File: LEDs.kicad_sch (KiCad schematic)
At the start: 62 parts, among them J5 Case Lighting

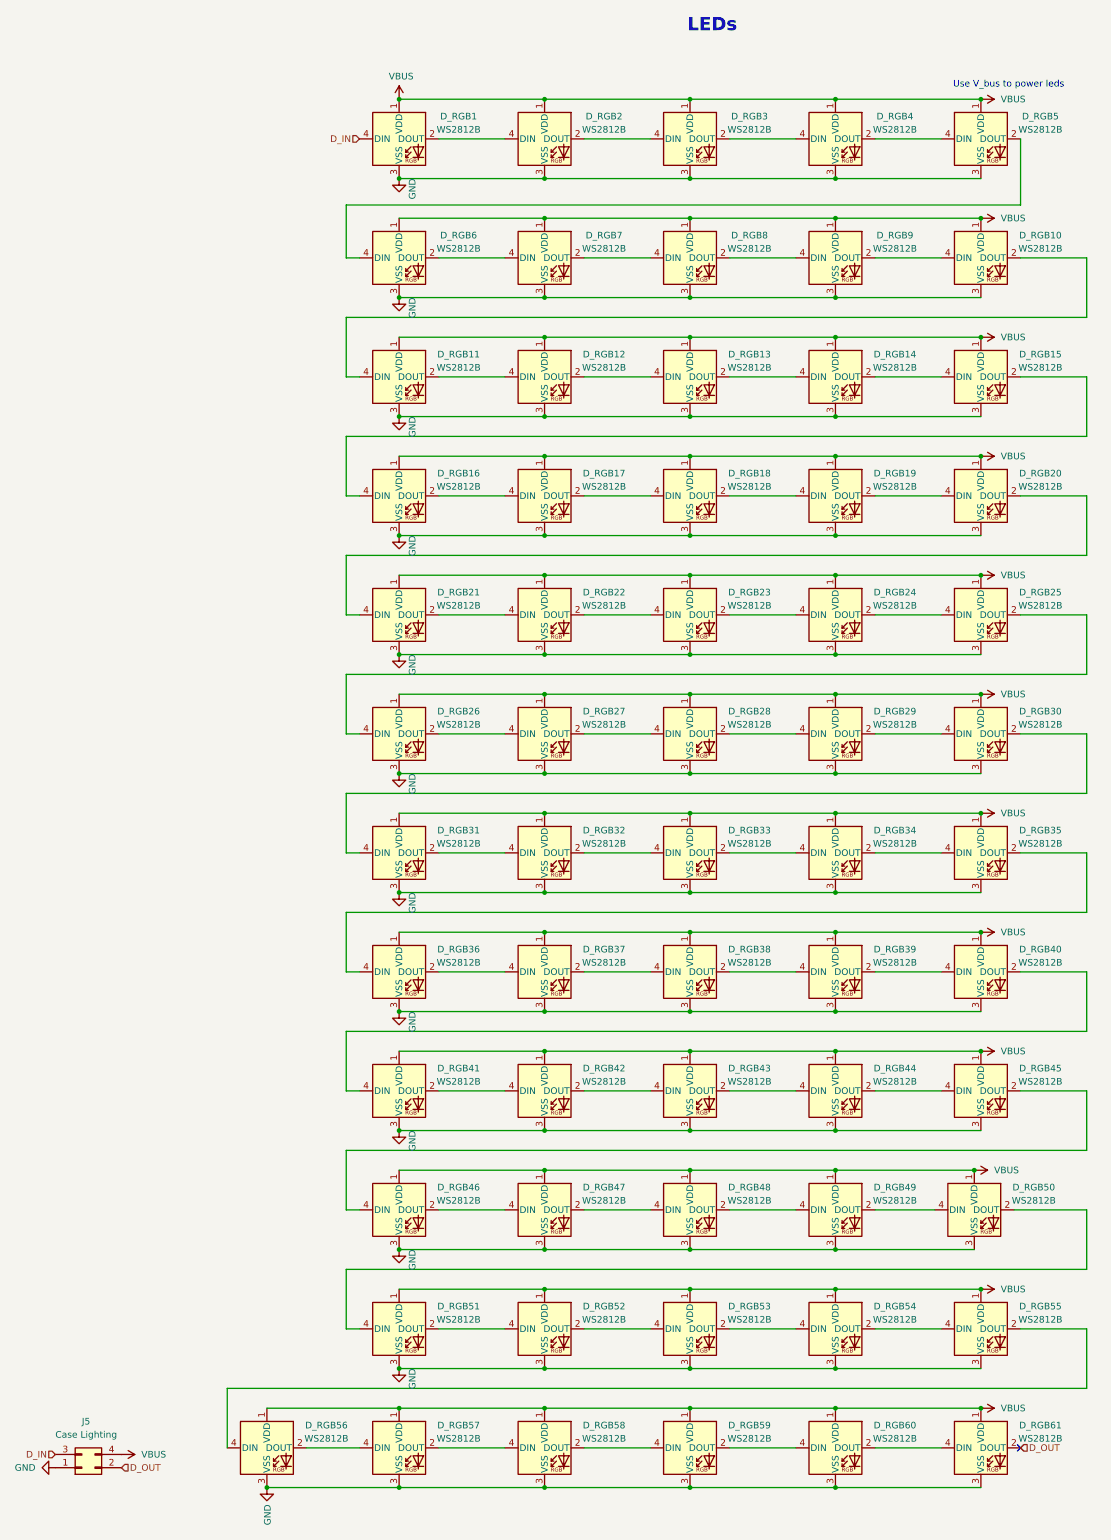
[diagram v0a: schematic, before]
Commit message: pretty much done
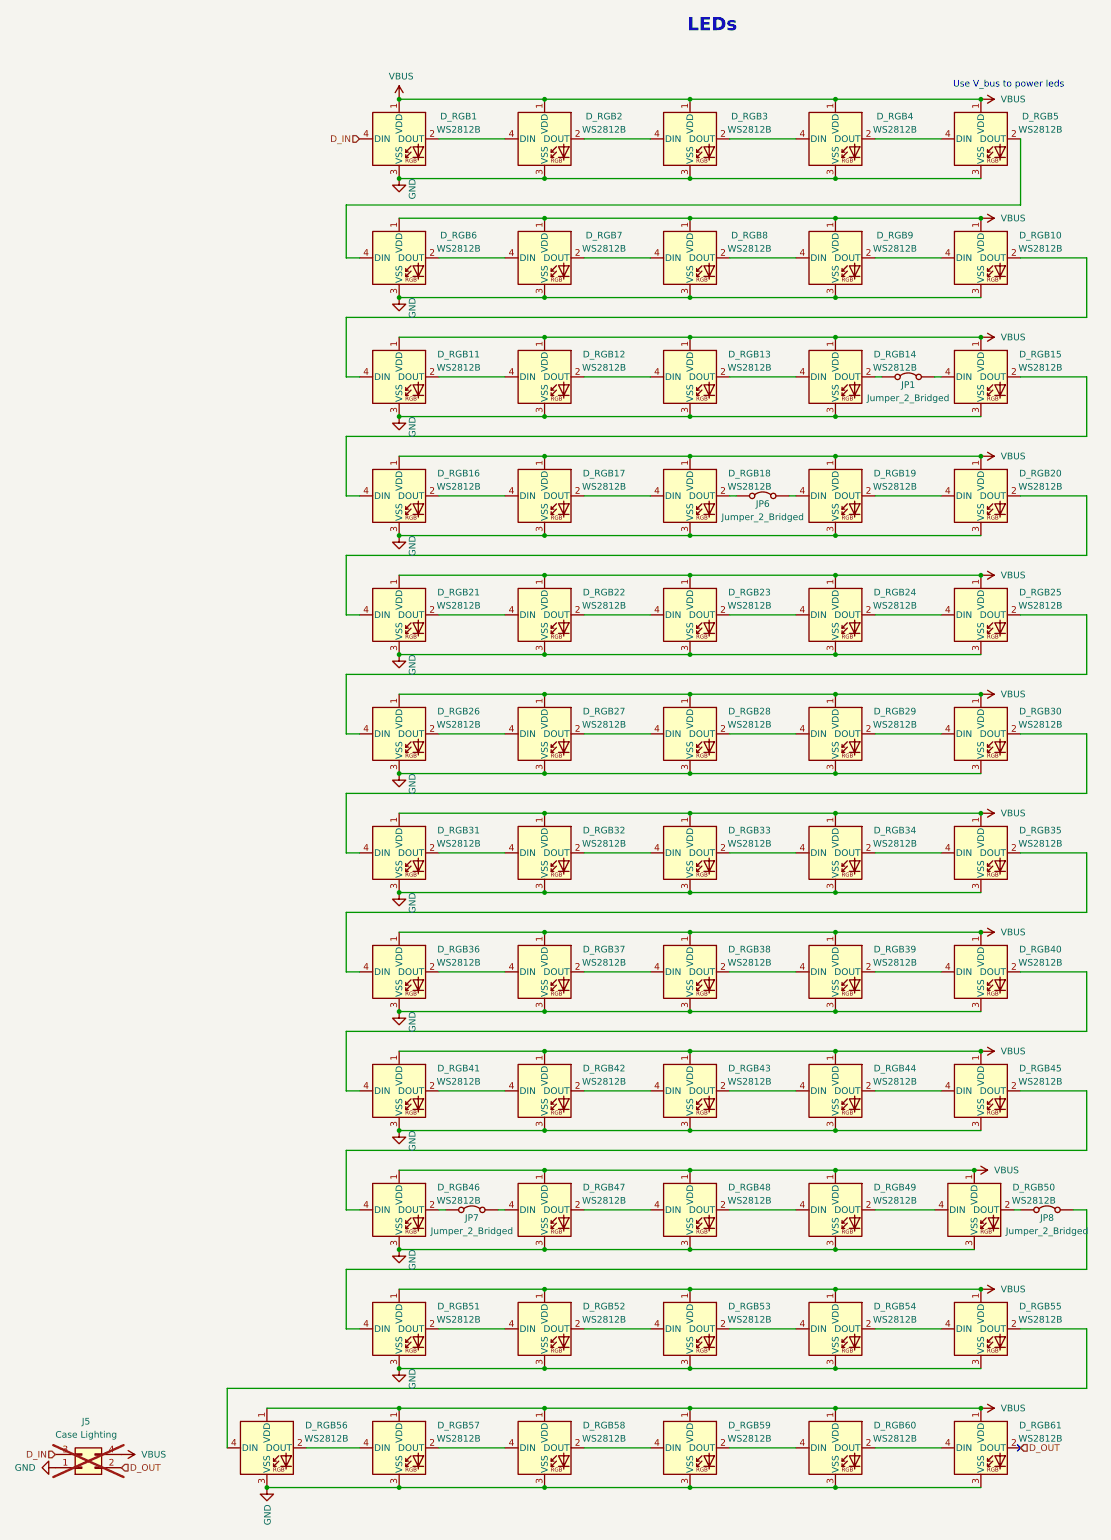
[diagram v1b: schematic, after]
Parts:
- added JP1, JP6, JP7, JP8: Jumper_2_Bridged, Jumper:SolderJumper-2_P1.3mm_Open_RoundedPad1.0x1.5mm, symbol Jumper:Jumper_2_Bridged
- J5: footprint Connector_JST:JST_PH_S4B-PH-K_1x04_P2.00mm_Horizontal -> Connector_PinHeader_2.54mm:PinHeader_1x04_P2.54mm_Vertical; now not fitted; now left out of the parts list
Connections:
- net at D_RGB14.2 (DOUT): now also JP1.1 (A); no longer D_RGB15.4 (DIN)
- net at D_RGB46.2 (DOUT): now also JP7.1 (A); no longer D_RGB47.4 (DIN)
- net at D_RGB50.2 (DOUT): now also JP8.1 (A); no longer D_RGB51.4 (DIN)
- net at D_RGB18.2 (DOUT): now also JP6.1 (A); no longer D_RGB19.4 (DIN)
- new net: D_RGB51.4 (DIN), JP8.2 (B)
- new net: D_RGB19.4 (DIN), JP6.2 (B)
- new net: D_RGB47.4 (DIN), JP7.2 (B)
- new net: D_RGB15.4 (DIN), JP1.2 (B)
